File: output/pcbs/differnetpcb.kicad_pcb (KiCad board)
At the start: 2 copper layers, 161.7 x 89.3 mm, 79 parts

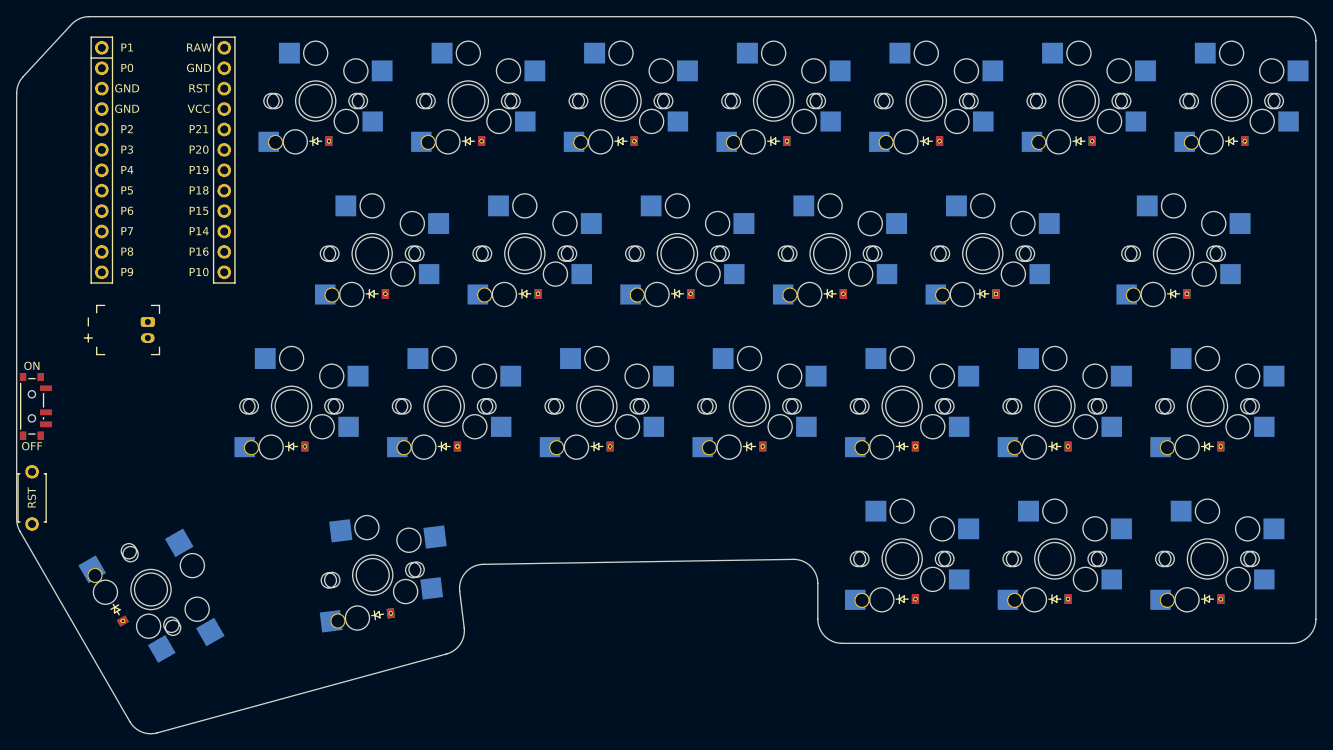
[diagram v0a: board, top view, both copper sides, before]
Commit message: some other commits
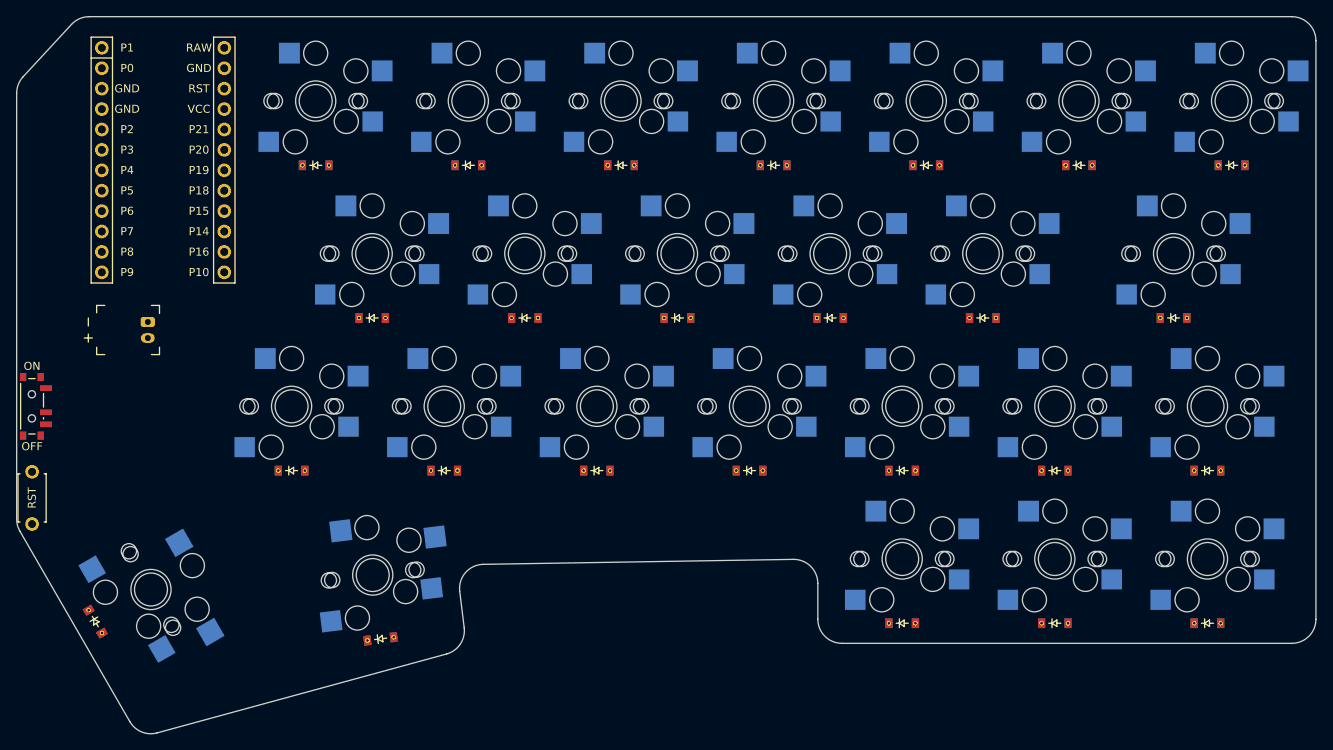
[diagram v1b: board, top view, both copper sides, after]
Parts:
- moved D1 3.00 mm to (150.0, 108.0)
- moved D10 3.00 mm to (195.0, 127.0)
- moved D11 3.00 mm to (214.0, 127.0)
- moved D12 3.00 mm to (233.0, 127.0)
- moved D13 3.00 mm to (256.8, 127.0)
- moved D14 3.00 mm to (147.0, 146.0)
- moved D15 3.00 mm to (166.0, 146.0)
- moved D16 3.00 mm to (185.0, 146.0)
- moved D17 3.00 mm to (204.0, 146.0)
- moved D18 3.00 mm to (223.0, 146.0)
- moved D19 3.00 mm to (242.0, 146.0)
- moved D2 3.00 mm to (169.0, 108.0)
- moved D20 3.00 mm to (261.0, 146.0)
- moved D21 3.00 mm to (223.0, 165.0)
- moved D22 3.00 mm to (242.0, 165.0)
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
